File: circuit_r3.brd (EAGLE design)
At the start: 160 x 100 mm, 25 parts, among them IC1 7805DT, U1 MCP4725, U2 MB85RC256VPF-G-JNERE2, U4 ATMEGA328P_VQFNVQFN, Y1 16MHz

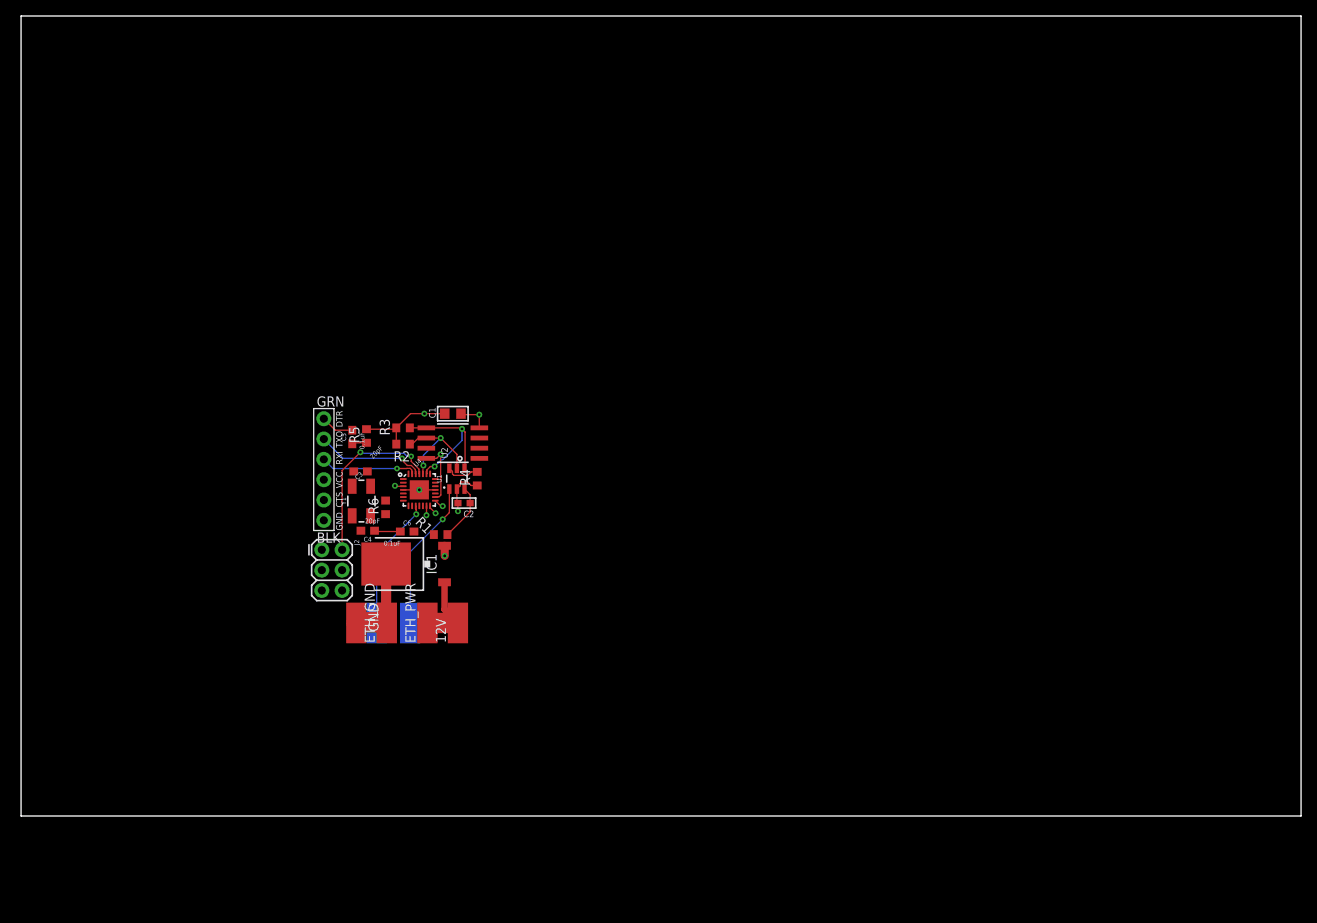
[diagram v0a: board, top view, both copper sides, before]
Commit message: Pretty good design.
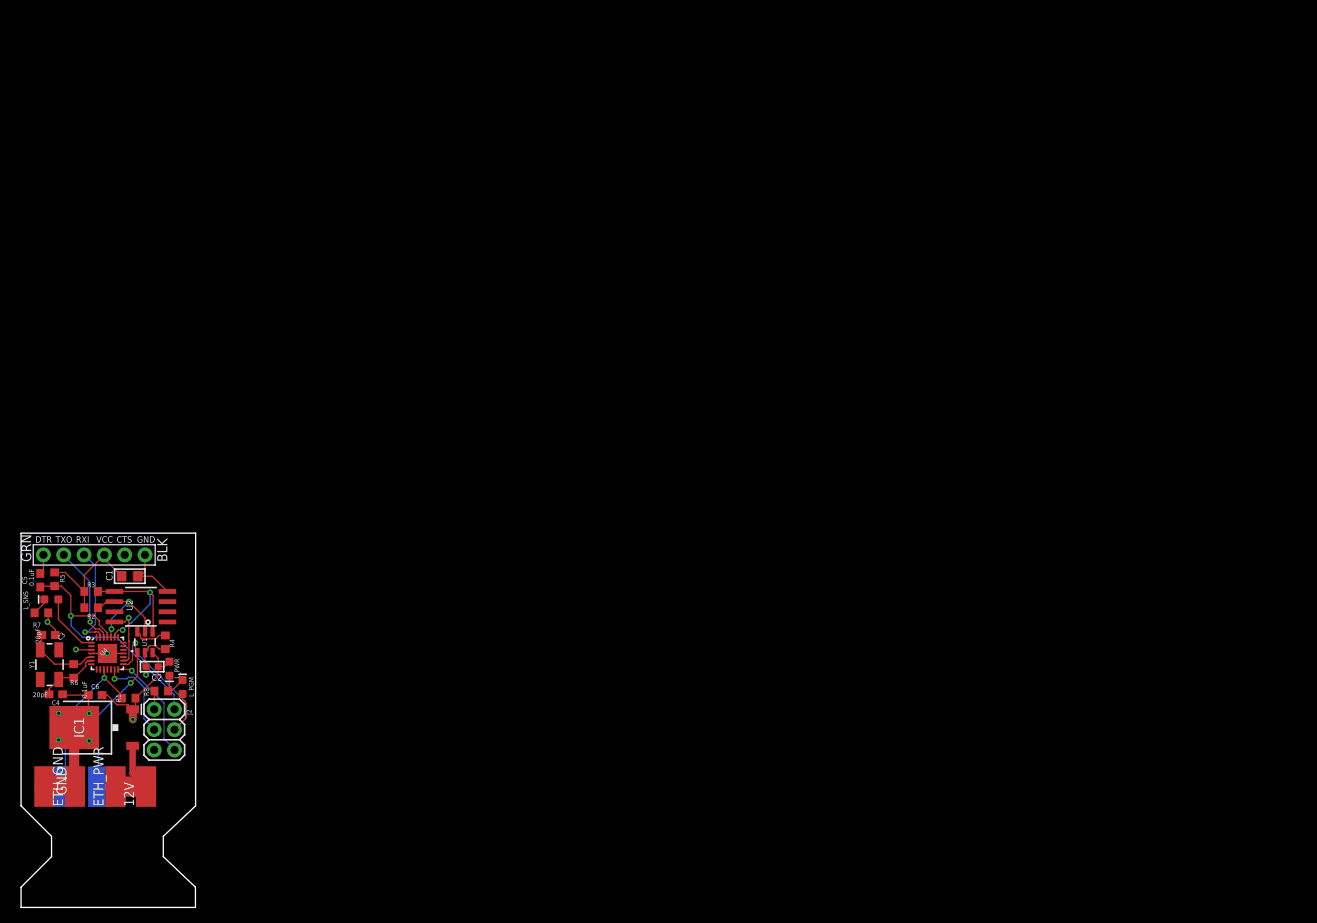
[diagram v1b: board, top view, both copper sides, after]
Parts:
- added L_PGM: GREEN, SparkFun-LED:LED-0603
- added L_PWR: RED, SparkFun-LED:LED-0603
- added L_SNS: BLUE, SparkFun-LED:LED-0603
- added R7, R8: 10k, adafruit:R0603
- moved C1 45.2 mm to (13.6, 30.0)
- moved C2 44.0 mm to (16.4, 18.7)
- moved C3 44.0 mm to (3.45, 22.6)
- moved ETH 44.0 mm to (5.46, 3.68)
- moved IC1 44.0 mm to (9.14, 11.0)
- moved R1 44.0 mm to (13.5, 14.7)
- moved R2 44.0 mm to (8.76, 26.0)
- moved R3 44.0 mm to (8.76, 28.1)
- moved R4 44.0 mm to (18.0, 21.7)
- moved U2 44.0 mm to (15.0, 26.2)
- moved U4 44.0 mm to (9.53, 19.1)
- moved Y1 44.0 mm to (3.56, 18.9)
- moved 12V 44.0 mm to (15.6, 3.68)
- moved C4 44.0 mm to (4.35, 15.2)
- moved C6 44.0 mm to (9.27, 15.1)
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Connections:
- new net LED_GND: L_PGM.C, L_PWR.C, R8.1
- new net N$2: L_SNS.C, R7.2
- new net SENS_IND: L_SNS.A, U4.1
- net GND: now also R7.1, R8.2
- net ISP_SCK: now also L_PGM.A
- net VCC: now also L_PWR.A
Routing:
- net ISP_SCK: track 1.20 -> 22.9 mm
- net GND: track 28.9 -> 43.8 mm, vias 3 -> 7
- net ISP_MISO: track 1.20 -> 13.9 mm
- net VCC: track 30.0 -> 42.1 mm, vias 4 -> 3
- net ISP_MOSI: track 1.18 -> 11.3 mm
- net XT1: track 0.00 -> 9.54 mm
- net RESET: track 24.1 -> 32.8 mm, vias 2 -> 1
- net SENS_IND: track 0.00 -> 7.82 mm
- net XT2: track 0.00 -> 7.68 mm
- net LED_GND: track 0.00 -> 4.38 mm
- net ETH: track 16.7 -> 20.2 mm
- net N$2: track 0.00 -> 2.18 mm
- net DTR: track 4.15 -> 2.48 mm
- net TXO: track 12.1 -> 13.4 mm
- net RXI: track 13.7 -> 12.7 mm
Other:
- board size 160 x 100 mm -> 21.8 x 46.8 mm
